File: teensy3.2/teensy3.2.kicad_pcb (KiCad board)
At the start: 2 copper layers, 31 parts, among them J1 USB_B_Micro, J2 Conn_01x26, J3 Conn_01x26, SW1 Prog, U1 LP38691SD-3.3, U2 MKL02Z32VFG4, U3 MK20DX256VLH7, Y1 32.768 KHz, Y2 16 MHz

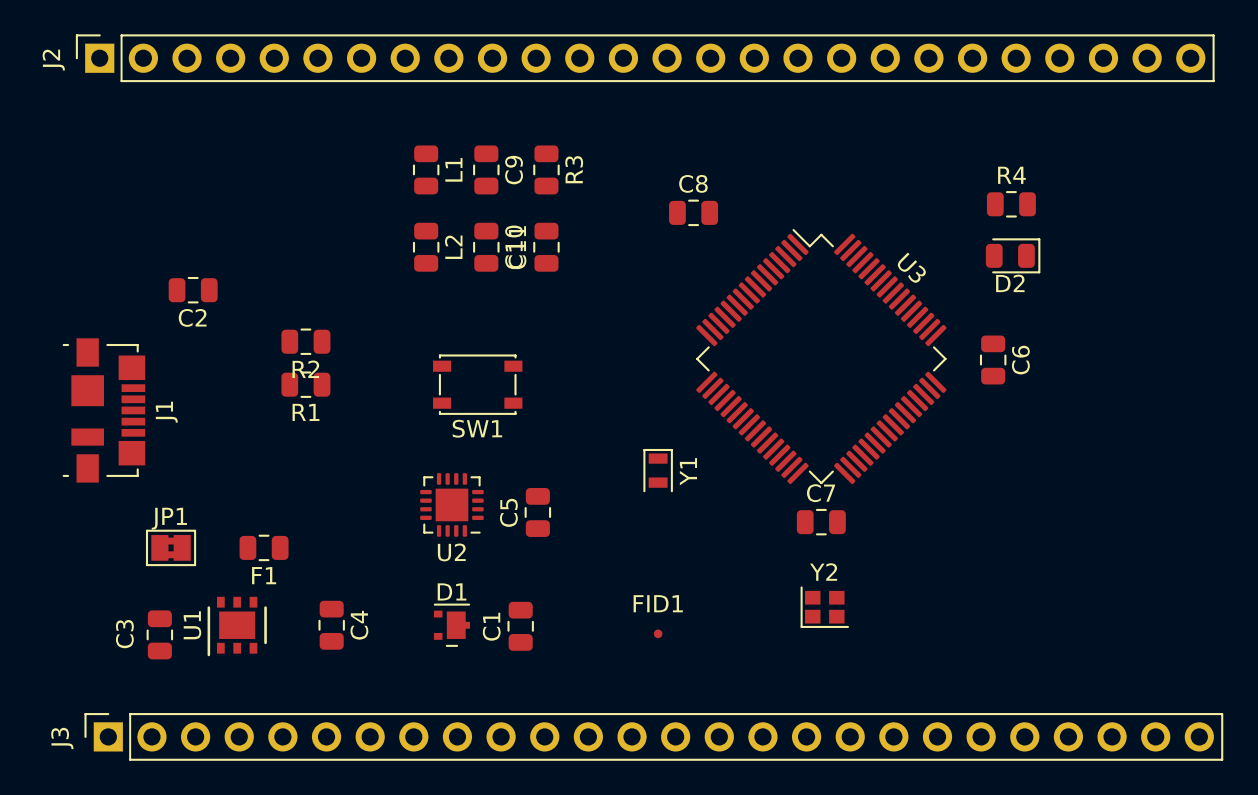
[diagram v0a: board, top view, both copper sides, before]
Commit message: avances pcb
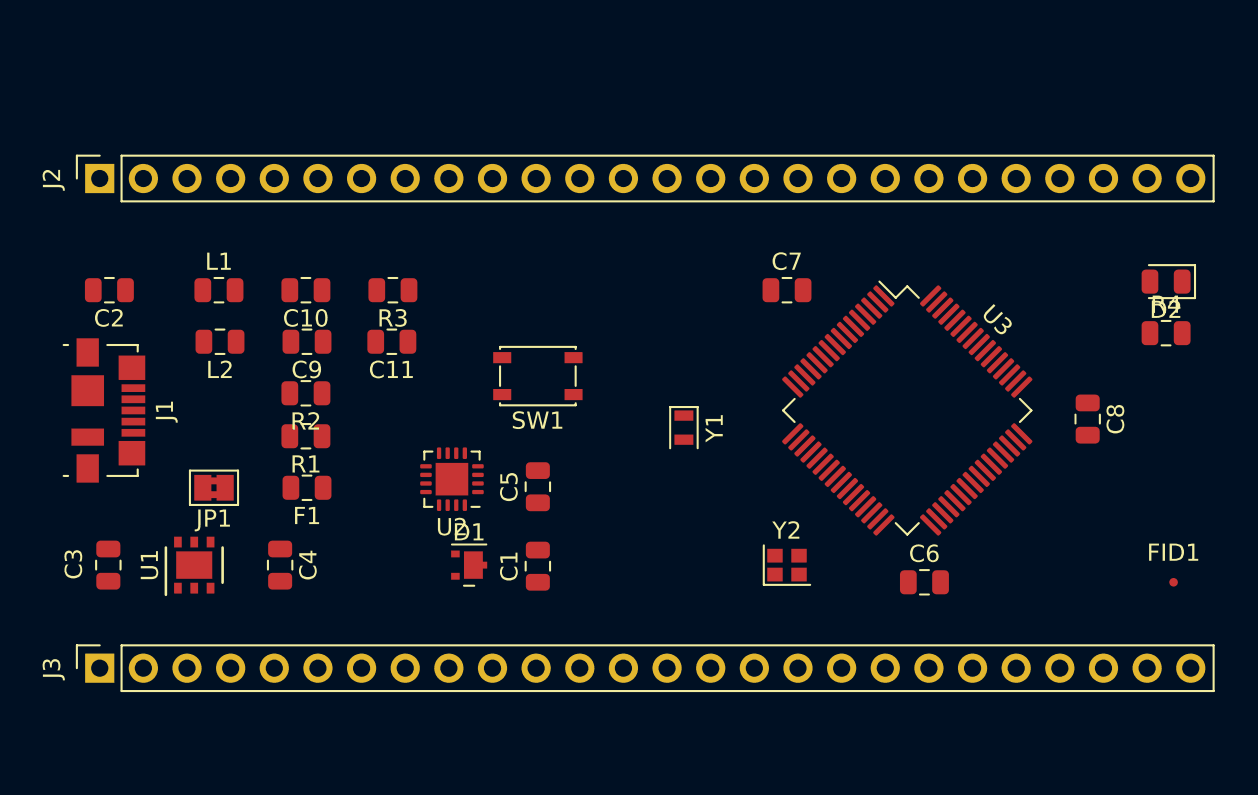
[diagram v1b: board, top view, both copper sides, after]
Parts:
- moved FID1 30.1 mm to (165.0, 103.0)
- moved C8 25.9 mm to (160.0, 93.5), turned to 270 degrees
- moved C9 14.5 mm to (114.6, 89.0), turned to 180 degrees
- moved L1 13.9 mm to (109.4, 86.0), turned to 0 degrees
- moved C7 13.6 mm to (142.5, 86.0)
- moved C6 13.5 mm to (150.5, 103.0), turned to 0 degrees
- moved L2 13.2 mm to (109.5, 89.0), turned to 180 degrees
- moved R4 11.7 mm to (164.6, 88.5)
- moved R3 11.4 mm to (119.6, 86.0), turned to 180 degrees
- moved C10 10.8 mm to (114.5, 86.0), turned to 180 degrees
- moved C11 10.5 mm to (119.5, 89.0), turned to 180 degrees
- moved D2 9.19 mm to (164.6, 85.5)
- moved J2 7.00 mm to (102.5, 79.5)
- moved U3 5.83 mm to (149.5, 93.0)
- moved C3 5.05 mm to (103.0, 102.0)
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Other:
- board text added: "Mínimos (Mayer 8 mils): Grillas: 0. 5mm, 0.25 mm Vía: 0.8 mm (0.4 mm) Margen: 0.18 mm Pista: 0.20 mm Dist. a borde: 0.30 mm Terminación: HASL"
